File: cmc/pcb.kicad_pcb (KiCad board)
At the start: 4 copper layers, 36.2 x 22 mm, 12 parts, among them J1 RJ45_LED, J2 RJ45_LED, U1 CMC, U11 CMC, U2 USBLC6-4SC6, U3 CMC, U4 CMC, U6 USBLC6-4SC6

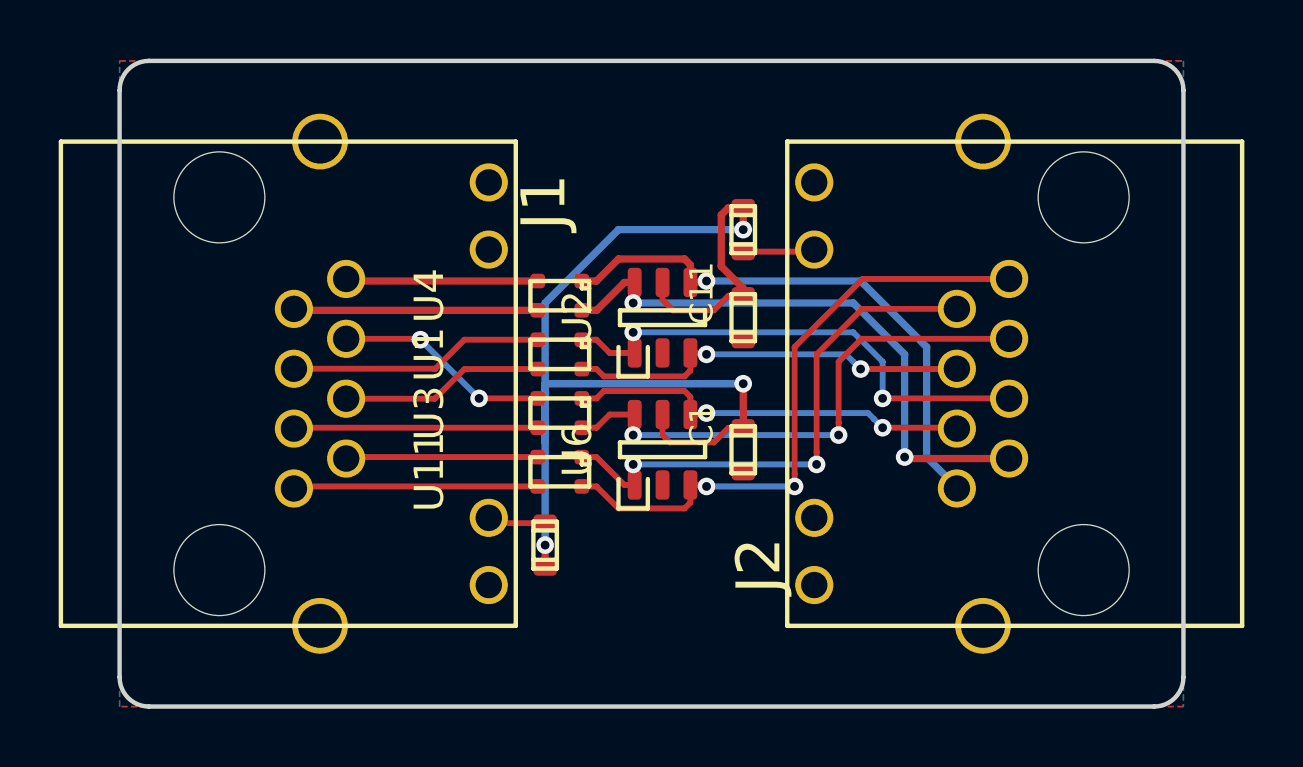
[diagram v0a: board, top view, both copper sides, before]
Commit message: jlc export
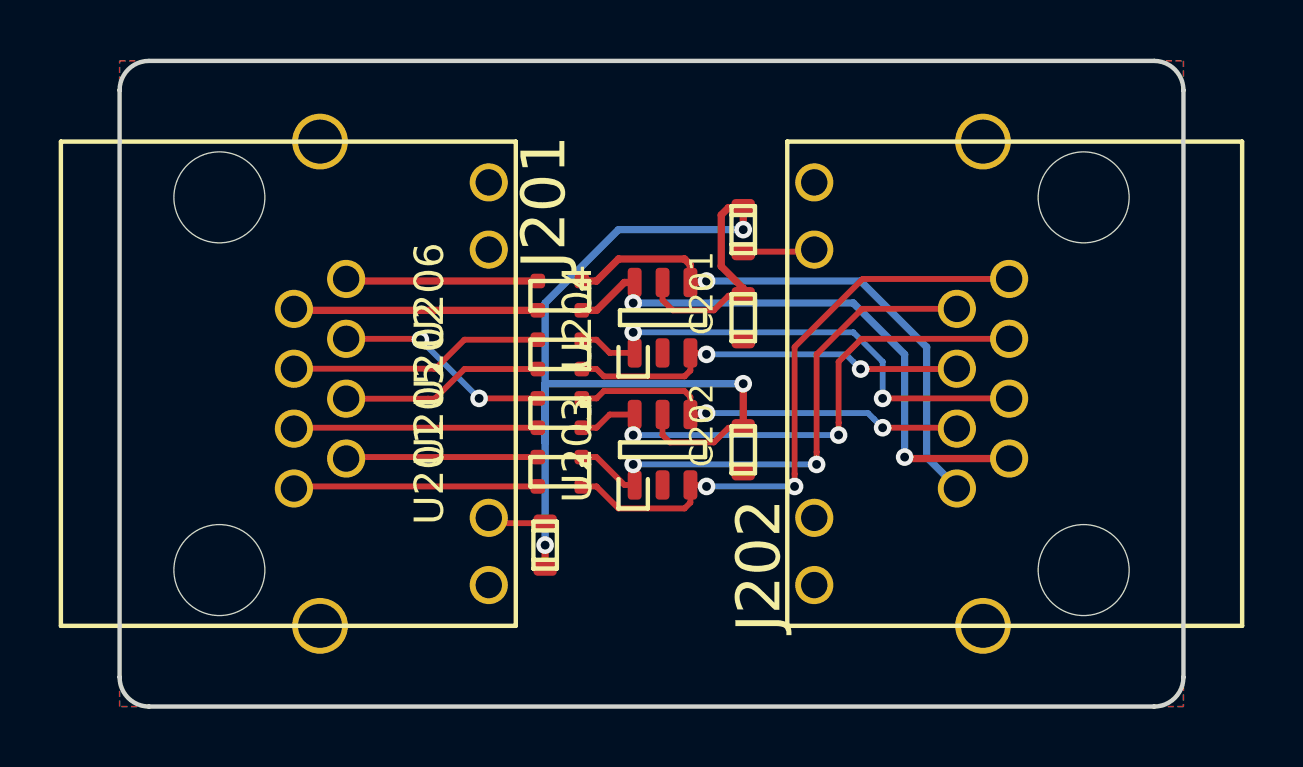
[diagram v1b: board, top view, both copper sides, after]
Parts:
- renumbered C11 to C201, C1 to C202, J1 to J201, J2 to J202, R1 to R201, R2 to R202, U11 to U201, U1 to U202, U6 to U203, U2 to U204, U3 to U205, U4 to U206
